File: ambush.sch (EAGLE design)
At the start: 130 parts, among them IC1 LM555N, IC10 LM555N, IC11 7430N, IC12 7400N, IC13 LM386N-3, IC14 74LS93N, IC15 74LS93N, IC16 7410N, IC17 7402N, IC18 7402N, IC19 7486N, IC2 7404N, IC20 74125N, IC21 7400N, IC22 LM555N, IC23 LM555N, IC24 7400N, IC25 LM555N, IC26 LM555N, IC27 74S20N, IC28 7404N, IC29 LM555N, IC3 LM555N, IC30 7400N, IC31 7475N, IC32 7485N, IC33 7485N, IC34 LM555N, IC35 LM555N, IC36 7402N, IC37 7404N, IC4 LM555N, IC5 7404N, IC6 74LS93N, IC7 LM555N, IC8 LM555N, IC9 74LS93N, T1 2N3904, T2 2N3904, T3 2N3904, T4 2N3904, T5 2N3904, T6 2N3904, Y1 14.3 MHz

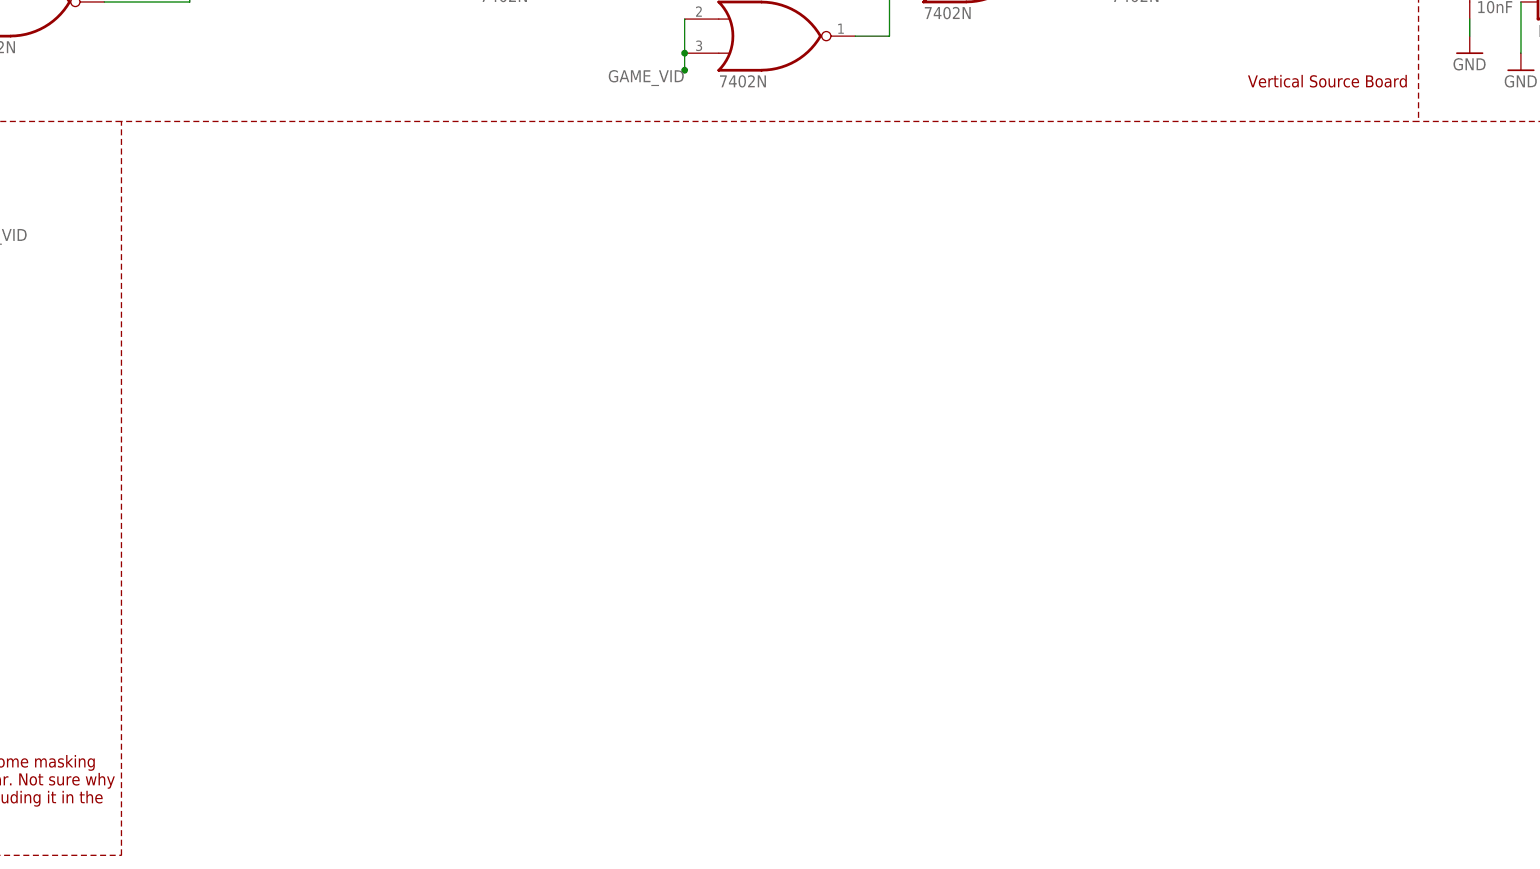
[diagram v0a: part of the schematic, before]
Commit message: -forgot to credit Heiserman
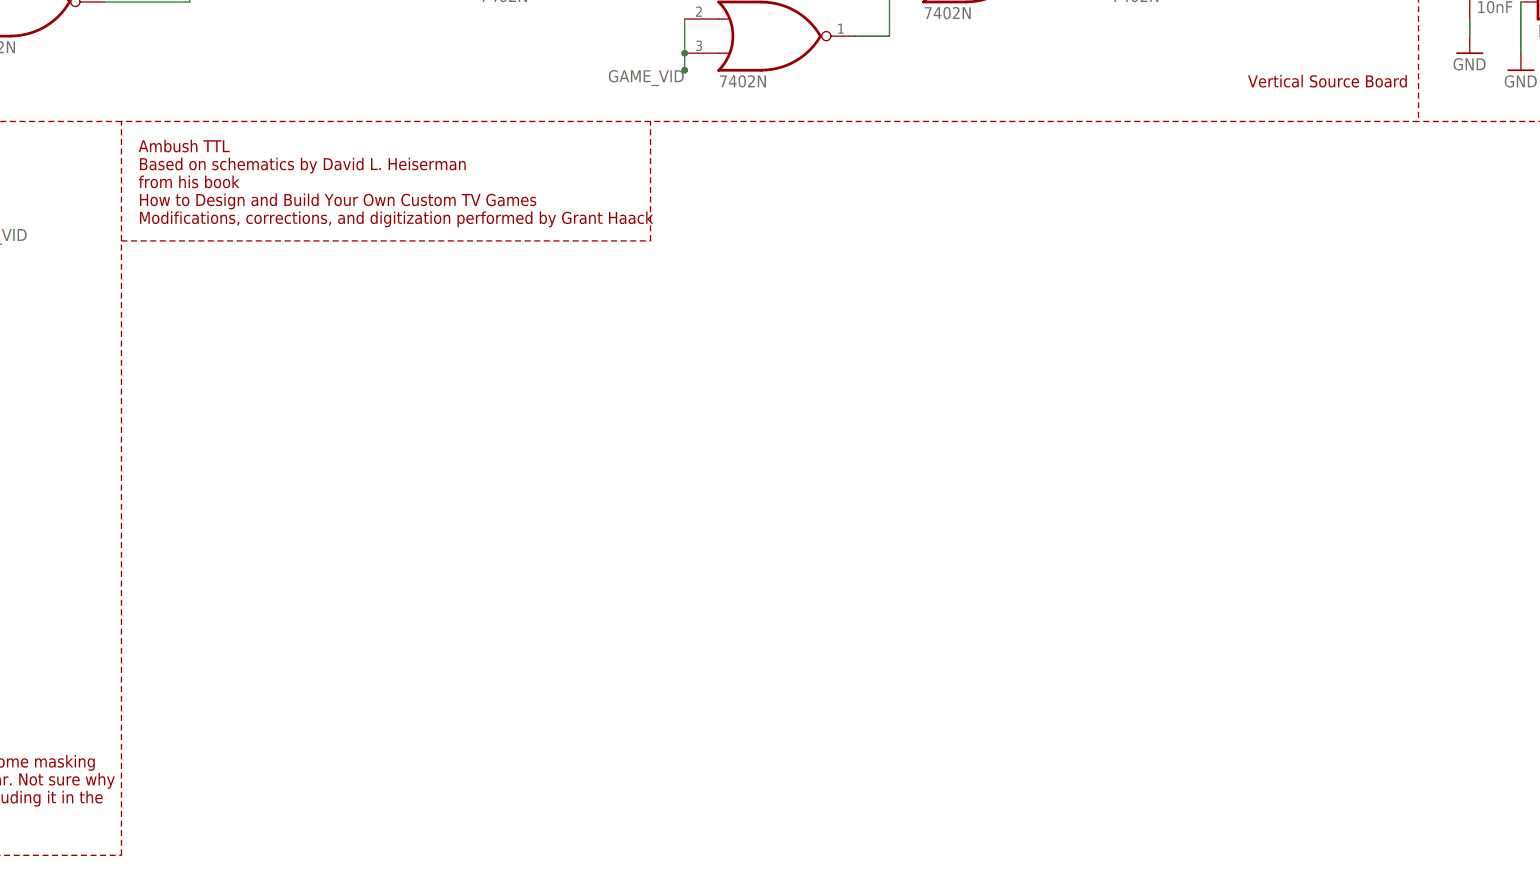
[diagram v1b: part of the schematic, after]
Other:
- note added: "Ambush TTL Based on schematics by David L. Heiserman from his book How to Design and Build Your Own Custom TV Games Modifications, corrections, and digitization performed by Grant Haack"
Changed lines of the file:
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@@
 <text x="528.32" y="-38.1" size="1.778" layer="94">Horizontal Source Board</text>
 <wire x1="642.62" y1="-40.64" x2="642.62" y2="-109.22" width="0.1524" layer="94" style="shortdash"/>
-<wire x1="642.62" y1="-109.22" x2="449.58" y2="-109.22" width="0.1524" layer="94" style="shortdash"/>
+<wire x1="642.62" y1="-109.22" x2="528.32" y2="-109.22" width="0.1524" layer="94" style="shortdash"/>
 <text x="617.22" y="-104.14" size="1.778" layer="94">Vertical Source Board</text>
+<wire x1="528.32" y1="-109.22" x2="449.58" y2="-109.22" width="0.1524" layer="94" style="shortdash"/>
 <wire x1="449.58" y1="-109.22" x2="342.9" y2="-109.22" width="0.1524" layer="94" style="shortdash"/>
 <wire x1="767.08" y1="71.12" x2="767.08" y2="-109.22" width="0.1524" layer="94" style="shortdash"/>
@@
 <wire x1="177.8" y1="-109.22" x2="177.8" y2="-218.44" width="0.1524" layer="94" style="shortdash"/>
 <wire x1="177.8" y1="-218.44" x2="449.58" y2="-218.44" width="0.1524" layer="94" style="shortdash"/>
-<wire x1="449.58" y1="-218.44" x2="449.58" y2="-109.22" width="0.1524" layer="94" style="shortdash"/>
+<wire x1="449.58" y1="-218.44" x2="449.58" y2="-127" width="0.1524" layer="94" style="shortdash"/>
 <text x="180.34" y="-215.9" size="1.778" layer="94">Figure Board</text>
+<text x="452.12" y="-124.46" size="1.778" layer="94">Ambush TTL
+Based on schematics by David L. Heiserman
+from his book
+How to Design and Build Your Own Custom TV Games
+Modifications, corrections, and digitization performed by Grant Haack</text>
+<wire x1="449.58" y1="-127" x2="449.58" y2="-109.22" width="0.1524" layer="94" style="shortdash"/>
+<wire x1="449.58" y1="-127" x2="528.32" y2="-127" width="0.1524" layer="94" style="shortdash"/>
+<wire x1="528.32" y1="-127" x2="528.32" y2="-109.22" width="0.1524" layer="94" style="shortdash"/>
 </plain>
 <instances>
